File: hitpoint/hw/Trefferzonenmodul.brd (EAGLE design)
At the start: 58.7 x 64.1 mm, 38 parts, among them X1 05-JST-B5B-XH-A, X2 05-JST-B5B-XH-A

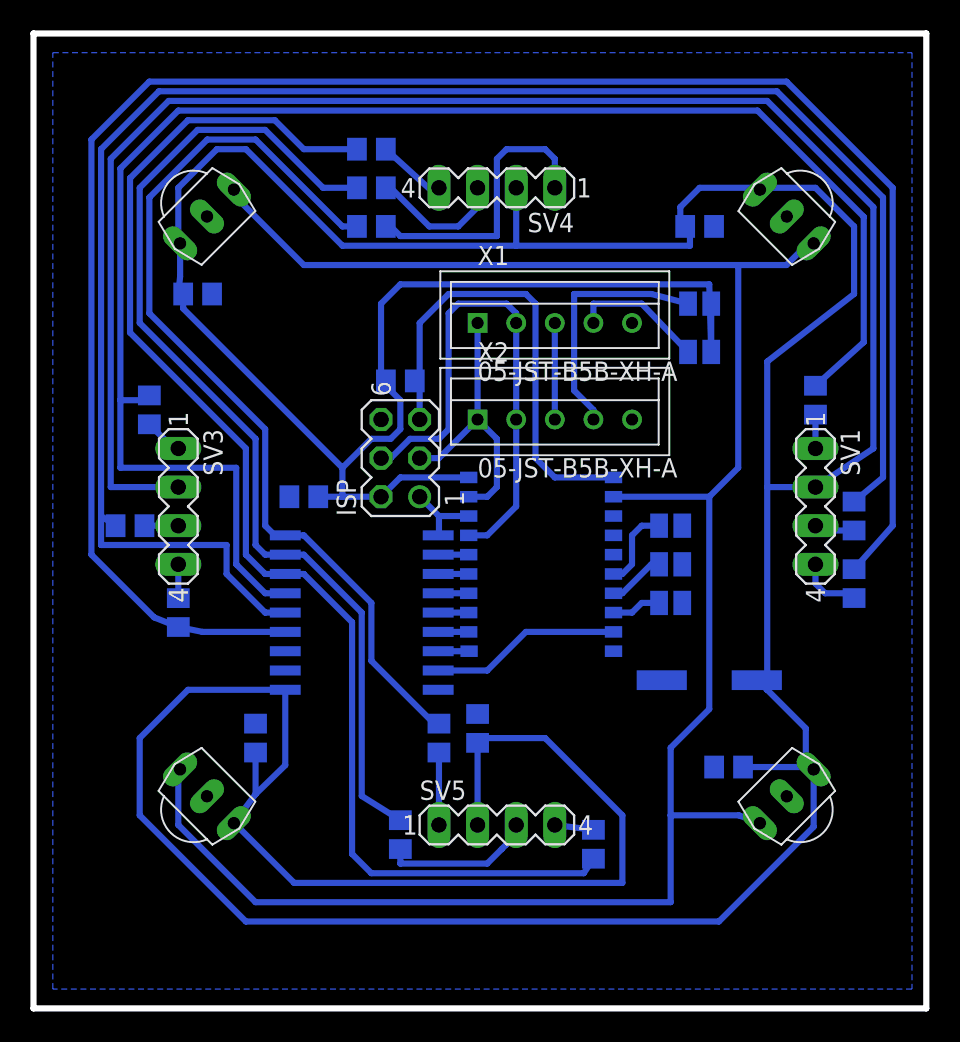
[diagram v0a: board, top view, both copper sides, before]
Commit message: neue platine
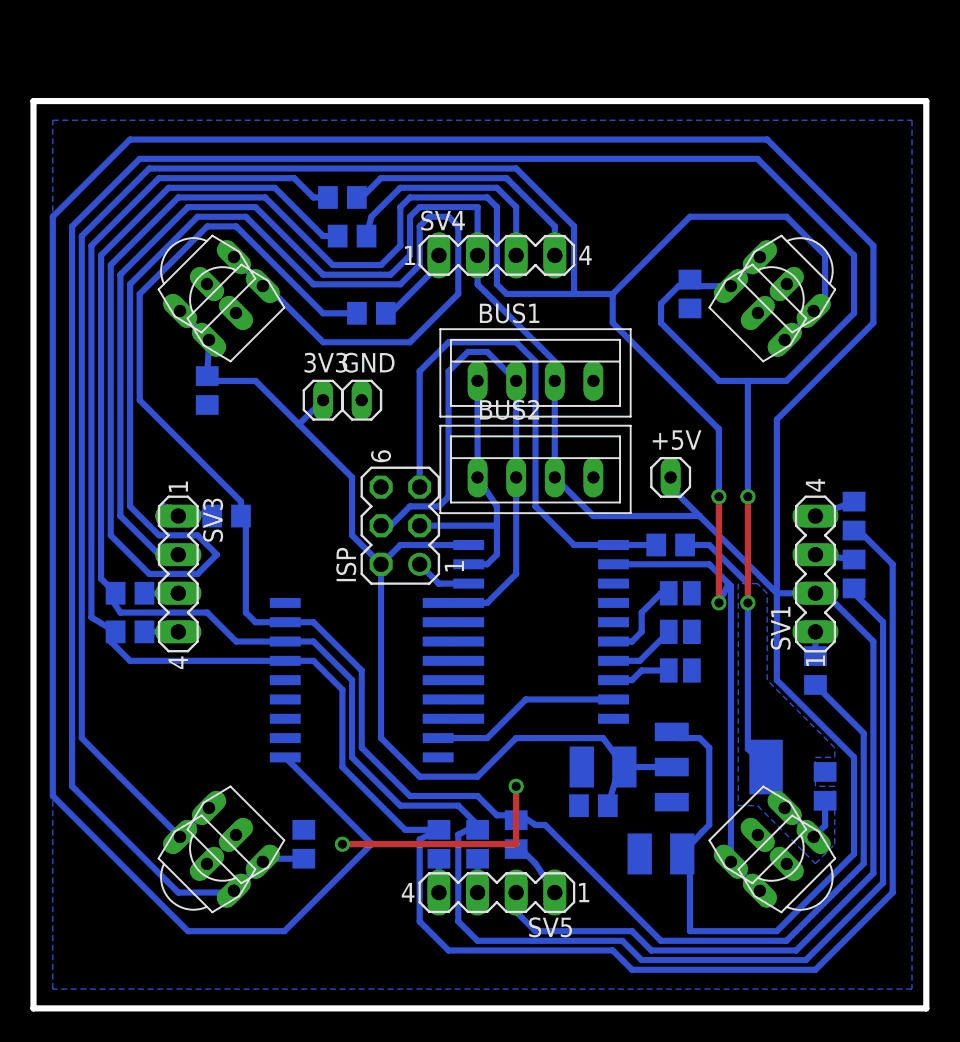
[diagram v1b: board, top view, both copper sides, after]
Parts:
- removed SJ4, SJ5: (no value), jumper:SJ
- removed X1, X2: 05-JST-B5B-XH-A, con-jst-xh:B5B-XH
- added +5V, 3V3, GND: (no value), wz:1X01
- added BUS1, BUS2: 04-JST-B4B-XH-A, wz:B4B-XH
- added LM1117: V_REG_MIC2920, wz:SOT223
- added U$5, U$6, U$7, U$8: TSOP1838, tsop:TSOP18XX
- C3: value 1000µ -> (none); device rcl:C0805 -> rcl:C1210
- C4: device rcl:UD-8X10_NICHICON -> rcl:C1210
- R13: value 1k -> 10k
- TINY2313A: device atmel:SO20L -> wz:SO20L
- moved C3 33.2 mm to (41.3, 10.2)
- moved R13 20.8 mm to (41.9, 30.5), turned to 0 degrees
- moved R10 17.8 mm to (51.4, 22.2), turned to 90 degrees
- moved R3 10.2 mm to (26.7, 10.8), turned to 270 degrees
- moved C1 9.16 mm to (36.8, 13.3), turned to 0 degrees
- moved C4 9.03 mm to (37.5, 15.9), turned to 0 degrees
- moved R7 8.64 mm to (12.7, 32.4), turned to 0 degrees
- moved R1 8.13 mm to (31.8, 11.4)
- moved C7 7.67 mm to (17.8, 10.8)
- moved C2 6.48 mm to (52.1, 14.6), turned to 90 degrees
- moved C8 6.38 mm to (11.4, 40.6), turned to 270 degrees
- moved R4 5.72 mm to (22.2, 45.7)
- moved R2 5.12 mm to (29.2, 10.8)
- moved SJ1 4.49 mm to (42.5, 22.2)
- moved SJ2 4.49 mm to (42.5, 24.8)
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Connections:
- removed net FREI: ULN2803.11
- removed net LED_B1: R3.1, R6.1, ULN2803.16
- removed net LED_B2: R12.1, R9.1, ULN2803.13
- removed net LED_G1: R2.1, R5.1, ULN2803.17
- removed net LED_G2: R11.1, R8.1, ULN2803.14
- removed net LED_R1: R1.1, R4.1, ULN2803.18
- removed net LED_R2: R10.1, R7.1, ULN2803.15
- removed net N$20: SJ4.1, X2.P$4
- removed net N$21: SJ5.1, X1.P$4
- removed net TINY_RX: TINY2313A.2, U$1.OUT, U$2.OUT, U$3.OUT, U$4.OUT
- removed net V_BATT: X1.P$3, X2.P$3
- new net +3V3: 3V3.1, C1.1, C2.1, C4.1, C6.1, C7.1, C8.1, ISP.2, LM1117.2, LM1117.4, R13.1, TINY2313A.20, U$1.VCC, U$2.VCC, U$3.VCC, U$4.VCC, U$5.VCC, U$6.VCC, U$7.VCC, U$8.VCC
- new net FREI1: ULN2803.18
- new net FREI5: ULN2803.14
- new net FREI6: ULN2803.13
- new net FREI7: ULN2803.12
- new net LED_B: R12.1, R3.1, R6.1, R9.1, ULN2803.15
- new net LED_G: R11.1, R2.1, R5.1, R8.1, ULN2803.16
- new net LED_R: R1.1, R10.1, R4.1, R7.1, ULN2803.17
- new net RX: TINY2313A.2, U$1.OUT, U$2.OUT, U$3.OUT, U$4.OUT, U$5.OUT, U$6.OUT, U$7.OUT, U$8.OUT
- net +5V: now also +5V.1, BUS1.P$3, BUS2.P$3, LM1117.3; no longer C1.1, C2.1, C4.+, C6.1, C7.1, C8.1, ISP.2, R13.1, SJ4.2, SJ5.2, TINY2313A.20, U$1.VCC, U$2.VCC, U$3.VCC, U$4.VCC
- net GND: now also BUS1.P$4, BUS2.P$4, C4.2, GND.1, LM1117.1, U$5.GND, U$6.GND, U$7.GND, U$8.GND; no longer C4.-, X1.P$5, X2.P$5
- net HAPTIK: now also ULN2803.11; no longer ULN2803.12
- net N$1: no longer ULN2803.1
- net SCL: now also BUS1.P$1, BUS2.P$1; no longer X1.P$1, X2.P$1
- net SDA: now also BUS1.P$2, BUS2.P$2, ULN2803.1; no longer X1.P$2, X2.P$2
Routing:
- net RX: track 0.00 -> 308.0 mm, vias 0 -> 2
- net +3V3: track 0.00 -> 250.9 mm, vias 0 -> 2
- net LED_B: track 0.00 -> 141.3 mm
- net TINY_RX: track 135.7 -> 0.00 mm
- net LED_G: track 0.00 -> 133.9 mm
- net LED_B2: track 125.1 -> 0.00 mm
- net LED_G2: track 119.1 -> 0.00 mm
- net LED_R: track 0.00 -> 110.5 mm
- net LED_R2: track 105.6 -> 0.00 mm
- net LED_B1: track 86.2 -> 0.00 mm
- net +5V: track 418.2 -> 349.0 mm
- net LED_G1: track 68.0 -> 0.00 mm
- net LED_R1: track 61.8 -> 0.00 mm
- net N$20: track 16.4 -> 0.00 mm
- net GND: track 0.00 -> 15.2 mm, vias 0 -> 2
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- added copper zone on layer 16, net +3V3
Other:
- board size 58.7 x 64.1 mm -> 58.7 x 59.7 mm
